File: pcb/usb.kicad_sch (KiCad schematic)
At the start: 2 parts, among them P1 USB_C_Plug_USB2.0

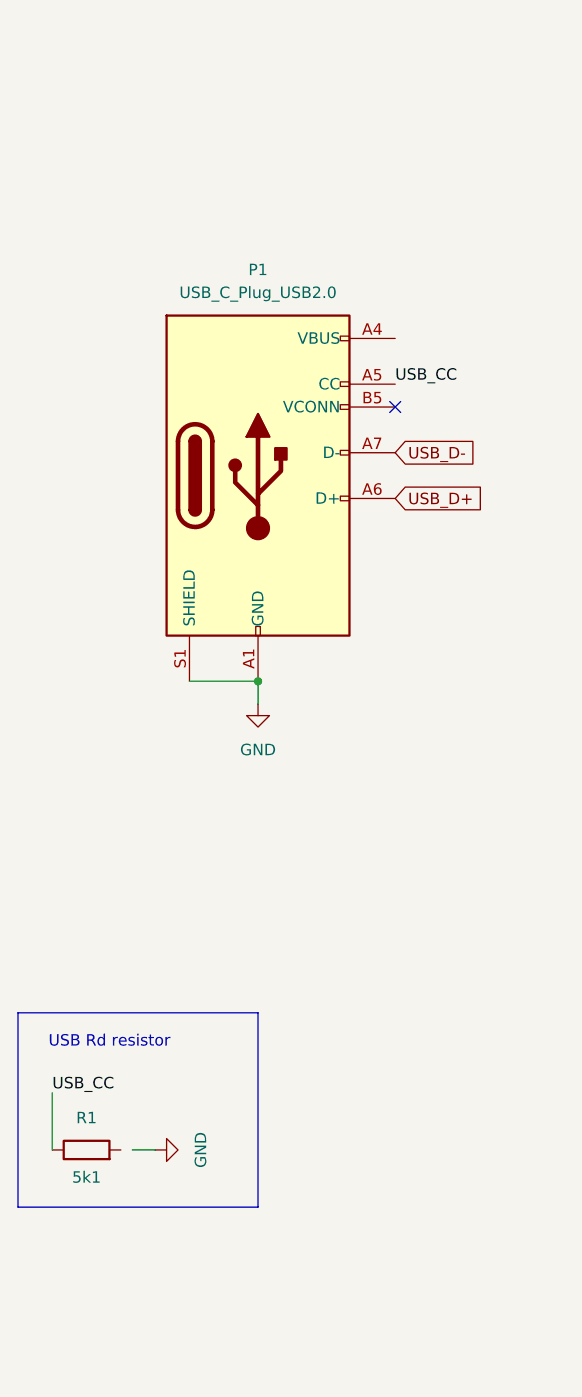
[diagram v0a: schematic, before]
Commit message: WIP: power / battery schematic 2
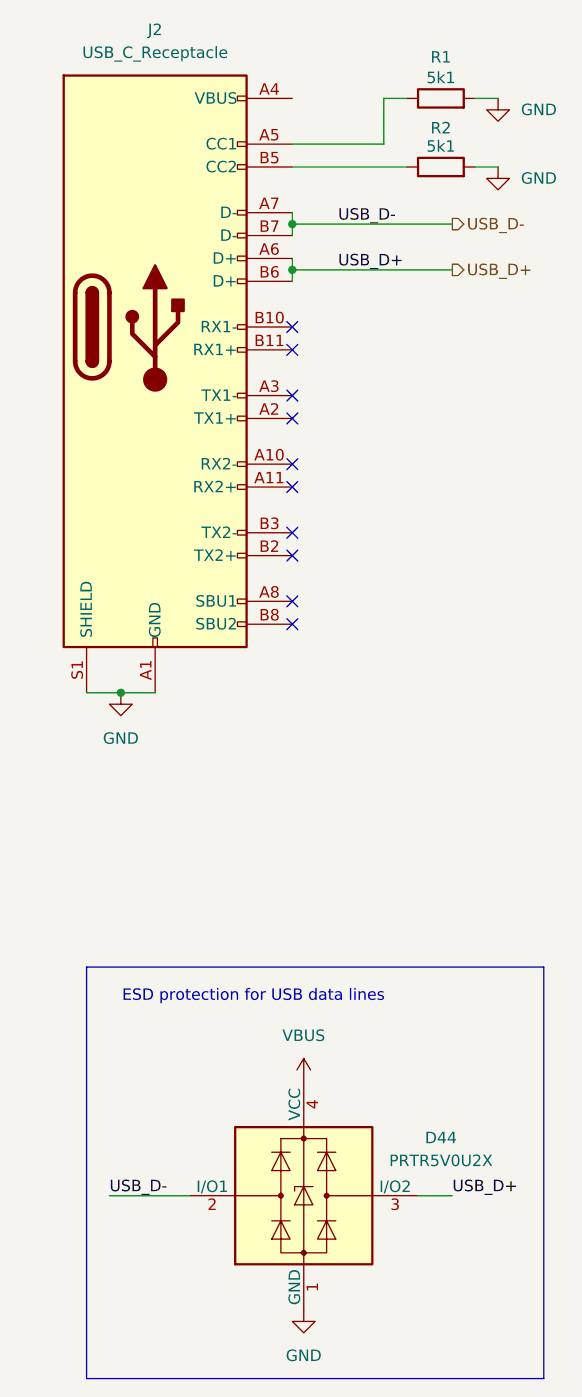
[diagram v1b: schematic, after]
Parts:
- removed P1: USB_C_Plug_USB2.0, symbol Connector:USB_C_Plug_USB2.0
- added D44: PRTR5V0U2X, Package_TO_SOT_SMD:SOT-143, symbol Power_Protection:PRTR5V0U2X
- added J2: USB_C_Receptacle, symbol Connector:USB_C_Receptacle
- added R2: 5k1, symbol Device:R
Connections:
- net GND: now also R1.2, D44.1 (GND), J2.A1 (GND), J2.A12 (GND), J2.B1 (GND), J2.B12 (GND), J2.S1 (SHIELD), R2.2
- net USB_D+: now also D44.3 (I/O2), J2.A6 (D+), J2.B6 (D+)
- net USB_D-: now also D44.2 (I/O1), J2.A7 (D-), J2.B7 (D-)
- net USB_CC: no longer names the net of R1.1
- net USB_CC: now also J2.A5 (CC1)
- new net: J2.A4 (VBUS), J2.A9 (VBUS), J2.B4 (VBUS), J2.B9 (VBUS)
- new net: J2.B5 (CC2), R2.1
- new net VBUS: D44.4 (VCC)
- no-connect marks 1 -> 10
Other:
- note added: "ESD protection for USB data lines"
- note removed: "USB Rd resistor"
- moved on the sheet: R1
